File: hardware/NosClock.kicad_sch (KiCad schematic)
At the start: 13 parts, among them U101 AMS1117-5, U102 К155ИД1

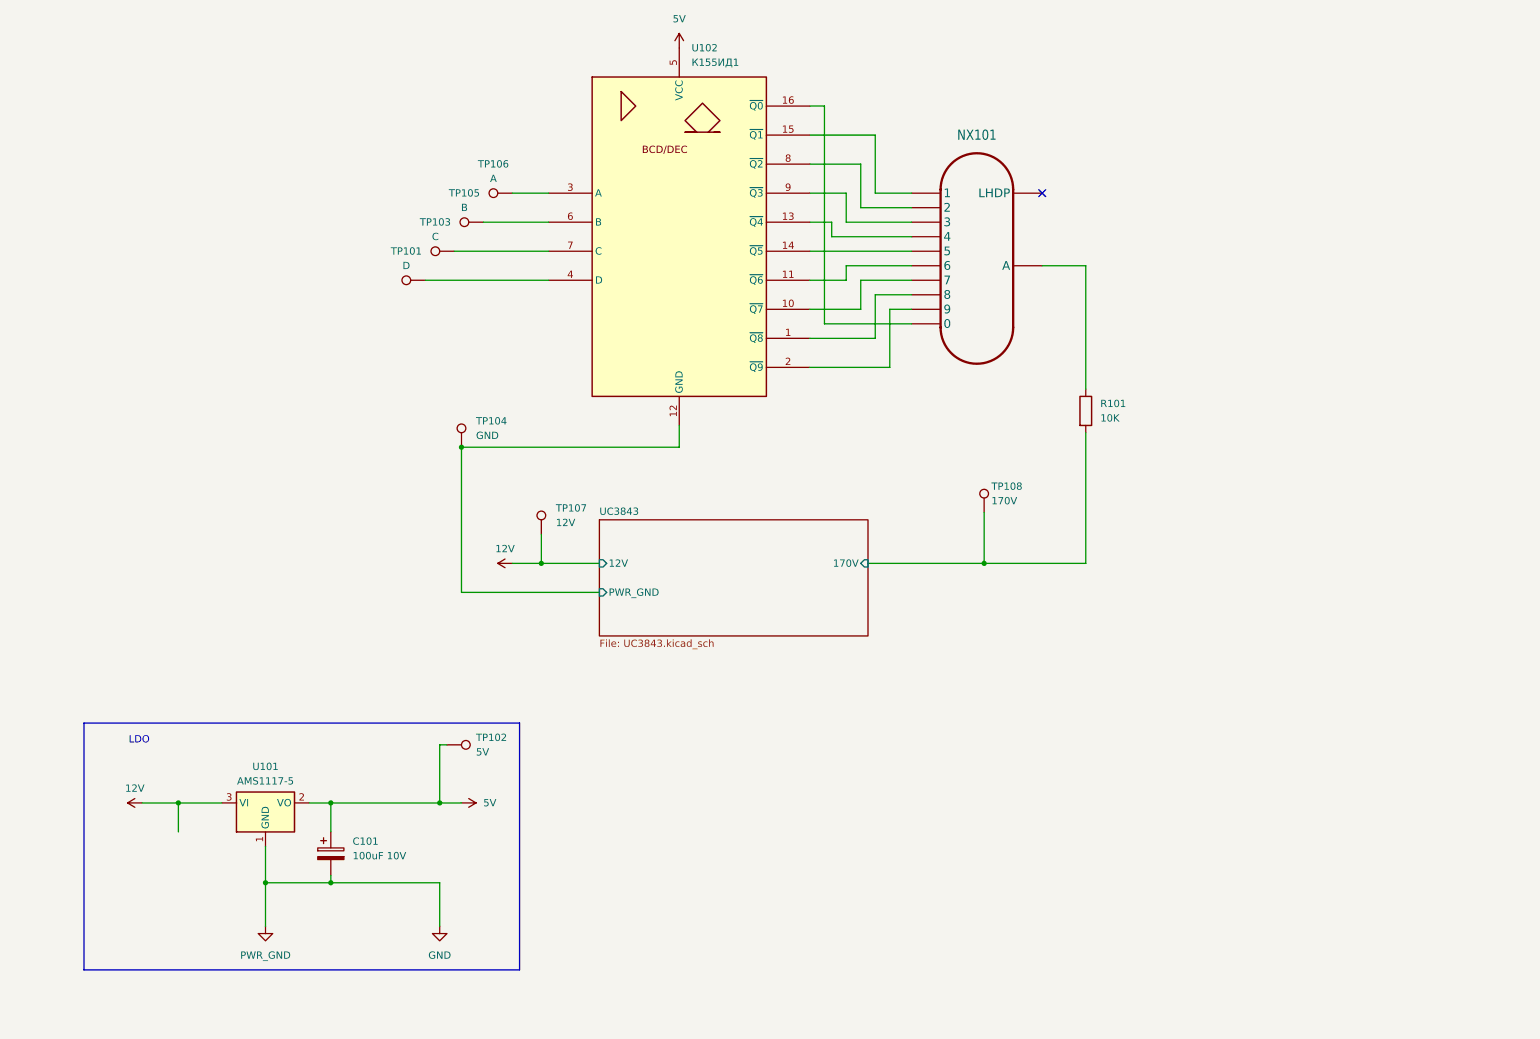
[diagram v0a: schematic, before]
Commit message: Lamps & 3.3v/5v
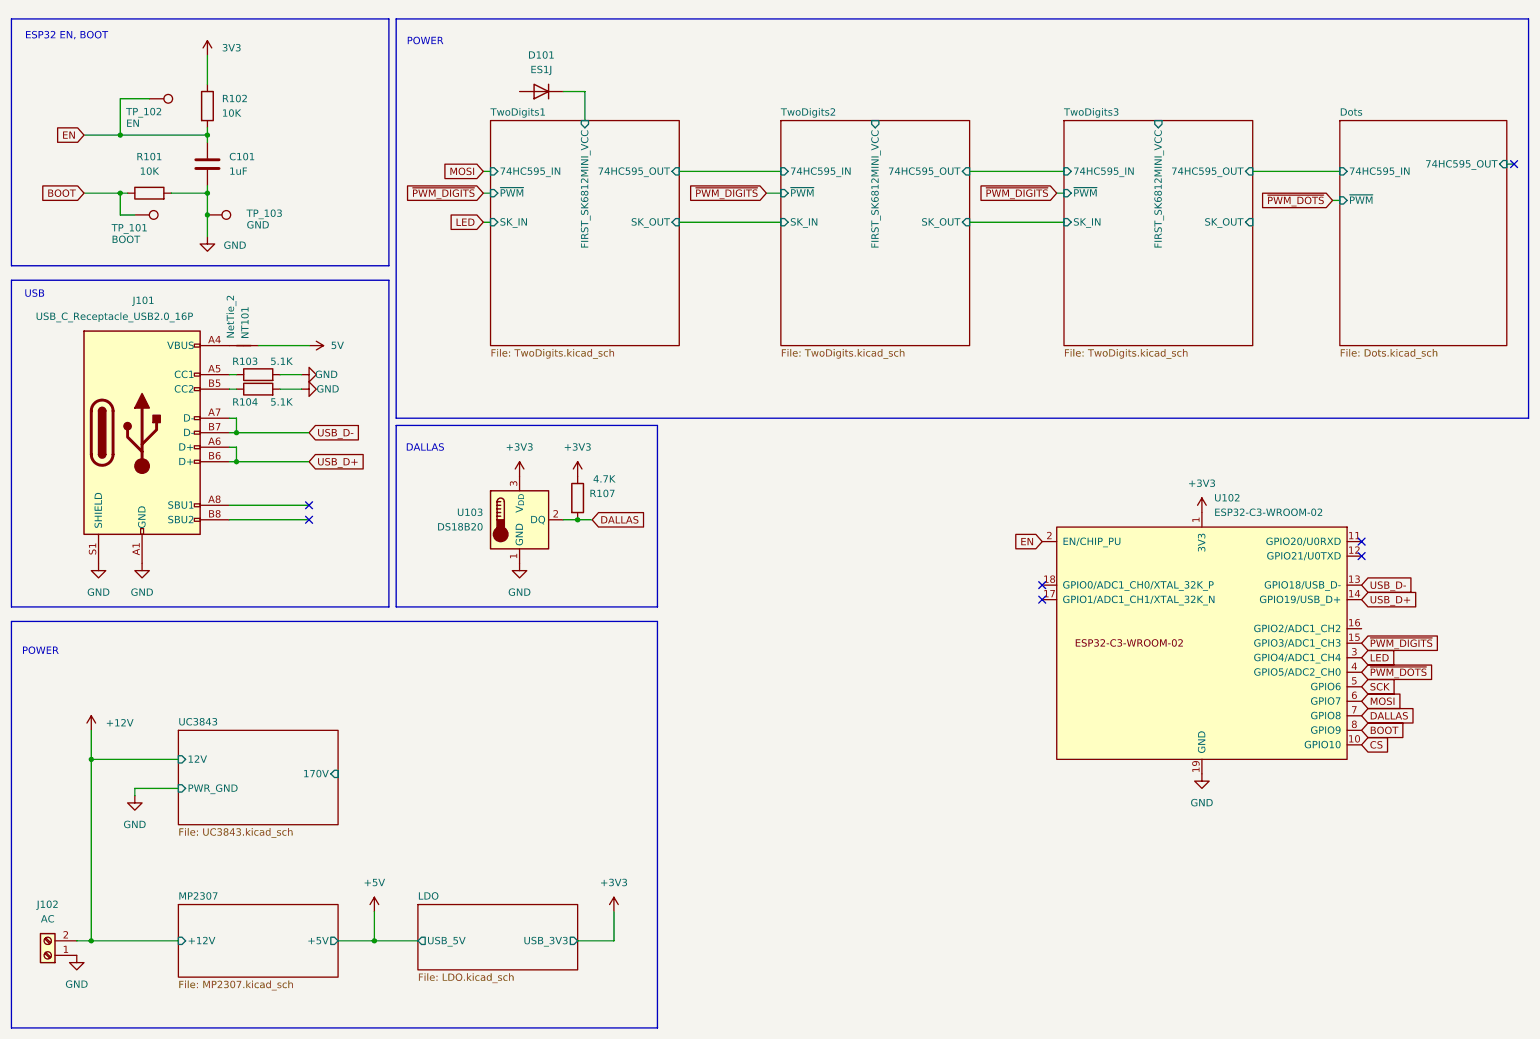
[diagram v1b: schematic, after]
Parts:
- removed C101: 100uF 10V, Capacitor_THT:CP_Radial_D6.3mm_P2.50mm, symbol Device:C_Polarized
- removed NX101: ~, nixies-us:nixies-us-IN-12-DSUB, symbol nixies-us:IN-12BORIGINAL
- removed TP101: D, TestPoint:TestPoint_Pad_3.0x3.0mm, symbol Connector:TestPoint
- removed TP102: 5V, TestPoint:TestPoint_Pad_3.0x3.0mm, symbol Connector:TestPoint
- removed TP103: C, TestPoint:TestPoint_Pad_3.0x3.0mm, symbol Connector:TestPoint
- removed TP104: GND, TestPoint:TestPoint_Pad_3.0x3.0mm, symbol Connector:TestPoint
- removed TP105: B, TestPoint:TestPoint_Pad_3.0x3.0mm, symbol Connector:TestPoint
- removed TP106: A, TestPoint:TestPoint_Pad_3.0x3.0mm, symbol Connector:TestPoint
- removed TP107: 12V, TestPoint:TestPoint_Pad_3.0x3.0mm, symbol Connector:TestPoint
- removed TP108: 170V, TestPoint:TestPoint_Pad_3.0x3.0mm, symbol Connector:TestPoint
- removed U101: AMS1117-5, Package_TO_SOT_SMD:SOT-223-3_TabPin2, symbol Regulator_Linear:AMS1117-3.3
- removed U102: К155ИД1, Package_DIP:DIP-16_W7.62mm, symbol 74xx_IEEE:74141
- added C101: 1uF, Capacitor_SMD:C_0805_2012Metric, symbol Device:C
- added D101: ES1J, Diode_SMD:D_SMA_Handsoldering, symbol Device:D
- added J101: USB_C_Receptacle_USB2.0_16P, Connector_USB:USB_C_Receptacle_HRO_TYPE-C-31-M-12, symbol Connector:USB_C_Receptacle_USB2.0_16P
- added J102: AC, NosLib:TerminalBlock_Phoenix_MKDS-1,5-2-5.08_1x02_P5.08mm_Horizontal, symbol Connector:Screw_Terminal_01x02
- added NT101: NetTie_2, NetTie:NetTie-2_SMD_Pad0.5mm, symbol Device:NetTie_2
- added R102: 10K, Resistor_SMD:R_0603_1608Metric, symbol Device:R
- added R103, R104: 5.1K, Resistor_SMD:R_0603_1608Metric, symbol Device:R
- added R107: 4.7K, Resistor_SMD:R_0603_1608Metric, symbol Device:R
- added TP_101: BOOT, NosLib:TestPoint_Pad_1.0x1.0mm, symbol Connector:TestPoint
- added TP_102: EN, NosLib:TestPoint_Pad_1.0x1.0mm, symbol Connector:TestPoint
- added TP_103: GND, NosLib:TestPoint_Pad_1.0x1.0mm, symbol Connector:TestPoint
- added U102: ESP32-C3-WROOM-02, PCM_Espressif:ESP32-C3-WROOM-02, symbol PCM_Espressif:ESP32-C3-WROOM-02
- added U103: DS18B20, Package_TO_SOT_THT:TO-92_Inline, symbol Sensor_Temperature:DS18B20
- R101: footprint Resistor_SMD:R_2512_6332Metric_Pad1.40x3.35mm_HandSolder -> Resistor_SMD:R_0603_1608Metric
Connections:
- net 5V: now also NT101.2
- net GND: now also R101.2, C101.2, J101.A1 (GND), J101.A12 (GND), J101.B1 (GND), J101.B12 (GND), J101.S1 (SHIELD), J102.1 (Pin_1), R103.2, R104.2, TP_103.1, U102.19 (GND), U102.9 (GND), U103.1 (GND)
- net UC3843/170V: no longer R101.2
- net BOOT: now reaches R101.1
- net BOOT: now also TP_101.1, U102.8 (GPIO9)
- new net: J101.A4 (VBUS), J101.A9 (VBUS), J101.B4 (VBUS), J101.B9 (VBUS), NT101.1
- new net: J101.A5 (CC1), R103.1
- new net: J101.B5 (CC2), R104.1
- new net +12V: J102.2 (Pin_2)
- new net +3V3: R107.1, U102.1 (3V3), U103.3 (V_{DD})
- new net 3V3: R102.1
- new net CS: U102.10 (GPIO10)
- new net DALLAS: R107.2, U102.7 (GPIO8), U103.2 (DQ)
- new net EN: C101.1, R102.2, TP_102.1, U102.2 (EN/CHIP_PU)
- new net LED: U102.3 (GPIO4/ADC1_CH4)
- new net MOSI: U102.6 (GPIO7)
- new net SCK: U102.5 (GPIO6)
- new net TwoDigits1/FIRST_SK6812MINI_VCC: D101.1 (K)
- new net USB_D+: J101.A6 (D+), J101.B6 (D+), U102.14 (GPIO19/USB_D+)
- new net USB_D-: J101.A7 (D-), J101.B7 (D-), U102.13 (GPIO18/USB_D-)
- new net ~{PWM_DIGITS}: U102.15 (GPIO3/ADC1_CH3)
- new net ~{PWM_DOTS}: U102.4 (GPIO5/ADC2_CH0)
- no-connect marks 1 -> 7
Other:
- added sheet Dots (Dots.kicad_sch)
- added sheet LDO (LDO.kicad_sch)
- added sheet MP2307 (MP2307.kicad_sch)
- added sheet TwoDigits1 (TwoDigits.kicad_sch)
- added sheet TwoDigits2 (TwoDigits.kicad_sch)
- added sheet TwoDigits3 (TwoDigits.kicad_sch)
- note added: "DALLAS"
- note added: "ESP32 EN, BOOT"
- note added: "POWER"
- note added: "USB"
- note removed: "LDO"
